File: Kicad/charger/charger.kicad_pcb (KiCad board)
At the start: 2 copper layers, 78 x 57 mm, 21 parts, among them K1 9V / 1A, K2 Battery, Q1 STN790A, U1 BQ2057W

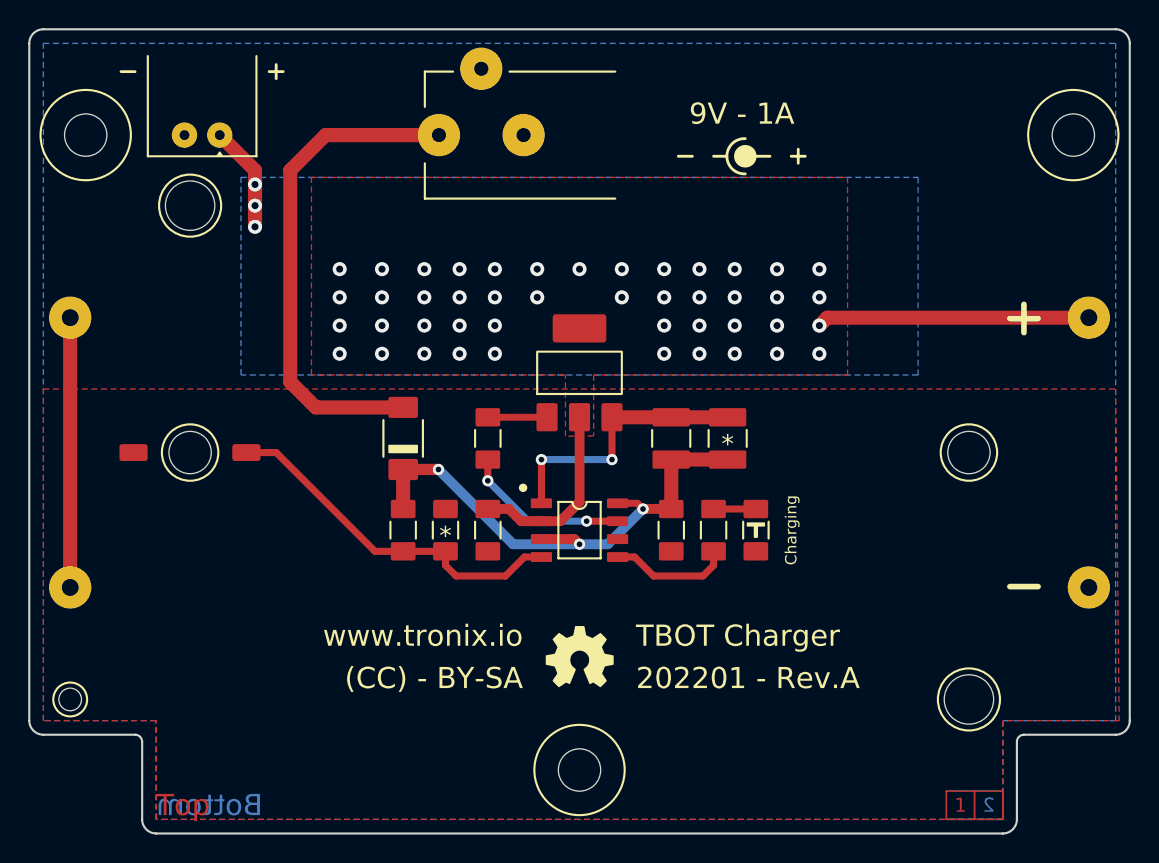
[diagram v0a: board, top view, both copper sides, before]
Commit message: Update
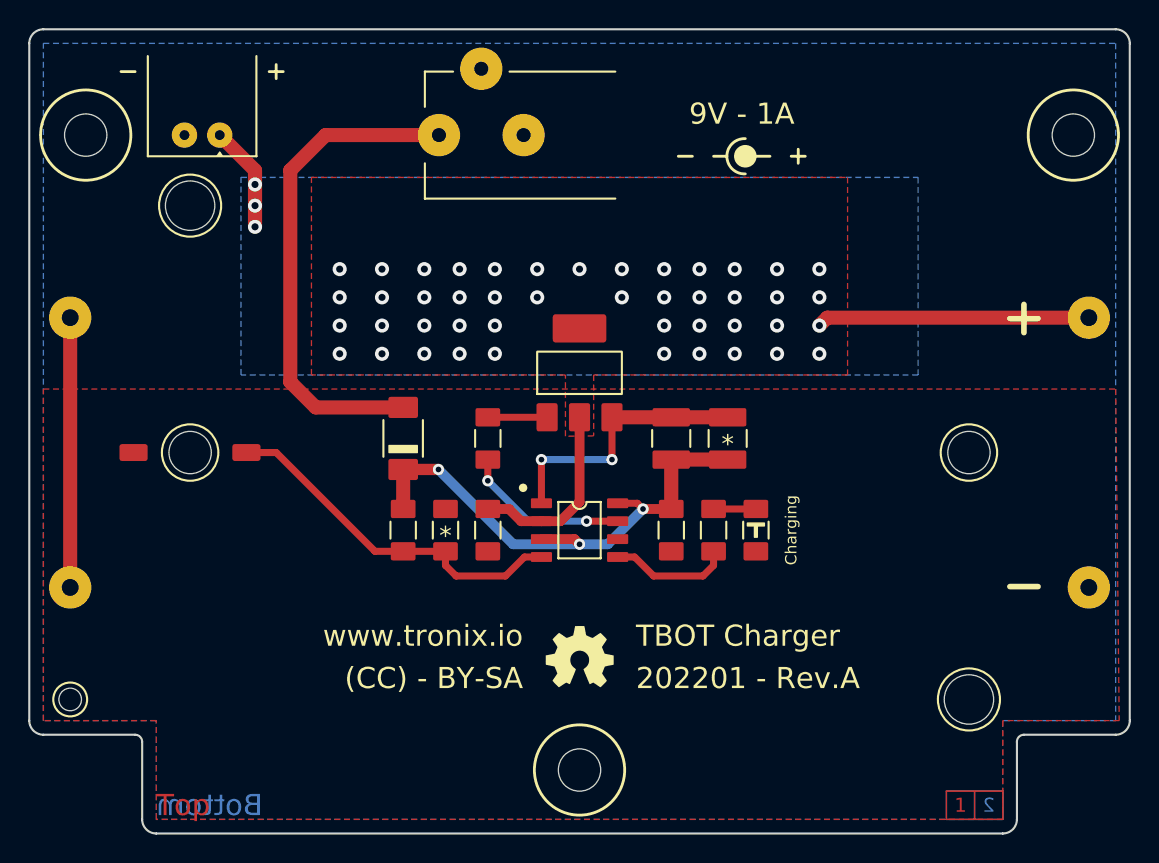
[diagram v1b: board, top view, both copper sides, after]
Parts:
- LED1: value PURPLE -> Charging
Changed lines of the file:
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@@
     (zone_connect 2)
     (attr smd)
-    (fp_text reference "D1" (at 4 0 90) (layer "F.Fab")
-        (effects (font (size 1 1) (thickness 0.15)))
-    )
-    (fp_text value "PMEG3030" (at 0 -2.5 90) (layer "F.Fab")
+    (fp_text reference "D1" (at 0 0 90) (layer "F.SilkS") hide
+        (effects (font (size 1 1) (thickness 0.15)))
+    )
+    (fp_text value "PMEG3030" (at 0 2.5 90) (layer "F.Fab")
         (effects (font (size 1 1) (thickness 0.15)))
     )
@@
     (zone_connect 2)
     (attr smd)
-    (fp_text reference "R6" (at 0 -2 -90) (layer "F.Fab")
+    (fp_text reference "R6" (at 0 -2 -90) (layer "F.SilkS") hide
         (effects (font (size 1 1) (thickness 0.15)))
     )
@@
     (zone_connect 2)
     (attr smd)
-    (fp_text reference "R5" (at 0 -2 90) (layer "F.Fab")
+    (fp_text reference "R5" (at 0 -2 90) (layer "F.SilkS") hide
         (effects (font (size 1 1) (thickness 0.15)))
     )
@@
     (property "ki_description" "Unpolarized Capacitor")
     (attr smd)
-    (fp_text reference "C1" (at 0 -2 -90) (layer "F.Fab")
+    (fp_text reference "C1" (at 0 -2 -90) (layer "F.SilkS") hide
         (effects (font (size 1 1) (thickness 0.15)))
     )
@@
     (zone_connect 2)
     (attr smd)
-    (fp_text reference "R1" (at 0 -2 -90) (layer "F.Fab")
+    (fp_text reference "R1" (at 0 -2 -90) (layer "F.SilkS") hide
         (effects (font (size 1 1) (thickness 0.15)))
     )
@@
     (property "ki_description" "DC Barrel Jack with an Internal Switch")
     (attr through_hole)
-    (fp_text reference "K1" (at 1 5.4625 180) (layer "F.Fab")
-        (effects (font (size 1 1) (thickness 0.15)))
-    )
-    (fp_text value "9V / 1A" (at -1 5.4625 180) (layer "F.Fab")
+    (fp_text reference "K1" (at 0 -2.5 90) (layer "F.SilkS") hide
+        (effects (font (size 1 1) (thickness 0.15)))
+    )
+    (fp_text value "9V / 1A" (at 0 15 90) (layer "F.Fab")
         (effects (font (size 1 1) (thickness 0.15)))
     )
@@
     (property "ki_description" "Unpolarized Capacitor")
     (attr smd)
-    (fp_text reference "C2" (at 0 -2 -90) (layer "F.Fab")
+    (fp_text reference "C2" (at 0 -2 -90) (layer "F.SilkS") hide
         (effects (font (size 1 1) (thickness 0.15)))
     )
@@
     (property "ki_description" "Medium current, high performance, low voltage PNP transistor")
     (attr smd)
-    (fp_text reference "Q1" (at 0 0 180) (layer "F.Fab")
-        (effects (font (size 1 1) (thickness 0.15)))
-    )
-    (fp_text value "STN790A" (at -4 0 180) (layer "F.Fab")
+    (fp_text reference "Q1" (at 0 -4.5 90) (layer "F.SilkS") hide
+        (effects (font (size 1 1) (thickness 0.15)))
+    )
+    (fp_text value "STN790A" (at 0 4.5 90) (layer "F.Fab")
         (effects (font (size 1 1) (thickness 0.15)))
     )
@@
     (property "ki_description" "Resistor")
     (attr smd)
-    (fp_text reference "R2" (at 0 -2.5 90) (layer "F.Fab")
+    (fp_text reference "R2" (at 0 -2.5 90) (layer "F.SilkS") hide
         (effects (font (size 1 1) (thickness 0.15)))
     )
@@
     (zone_connect 2)
     (attr smd)
-    (fp_text reference "TH1" (at 0 -3.81 180) (layer "F.Fab")
-        (effects (font (size 1 1) (thickness 0.15)))
-    )
-    (fp_text value "10k" (at 0 3.81 180) (layer "F.Fab")
+    (fp_text reference "TH1" (at 0 -3 180) (layer "F.SilkS") hide
+        (effects (font (size 1 1) (thickness 0.15)))
+    )
+    (fp_text value "10k" (at 0 3 180) (layer "F.Fab")
         (effects (font (size 1 1) (thickness 0.15)))
     )
@@
     (zone_connect 2)
     (attr smd)
-    (fp_text reference "LED1" (at 0 -2 90) (layer "F.Fab")
-        (effects (font (size 1 1) (thickness 0.15)))
-    )
-    (fp_text value "PURPLE" (at 0 2 90) (layer "F.Fab")
+    (fp_text reference "LED1" (at 0 -2 90) (layer "F.SilkS") hide
+        (effects (font (size 1 1) (thickness 0.15)))
+    )
+    (fp_text value "Charging" (at 0 2 90) (layer "F.Fab")
         (effects (font (size 1 1) (thickness 0.15)))
     )
@@
     (property "ki_keywords" "538-22-05-7025 / 538-50-37-5023 / 538-08-70-1039-CT")
     (attr through_hole)
-    (fp_text reference "K2" (at -0.5 -4.5) (layer "F.Fab")
-        (effects (font (size 1 1) (thickness 0.15)))
-    )
-    (fp_text value "Battery" (at -0.5 -3) (layer "F.Fab")
+    (fp_text reference "K2" (at -1.5 -8) (layer "F.SilkS") hide
+        (effects (font (size 1 1) (thickness 0.15)))
+    )
+    (fp_text value "Battery" (at -1.5 3) (layer "F.Fab")
+        (effects (font (size 1 1) (thickness 0.15)))
+    )
+    (fp_text user "1" (at 2 0.2) (layer "F.Fab")
         (effects (font (size 1 1) (thickness 0.15)))
     )
     (fp_text user "${REFERENCE}" (at -1.25 -8) (layer "F.Fab")
-        (effects (font (size 1 1) (thickness 0.15)))
-    )
-    (fp_text user "1" (at 1.9 0.1 unlocked) (layer "F.Fab")
         (effects (font (size 1 1) (thickness 0.15)))
     )
@@
     (property "ki_description" "Resistor")
     (attr smd)
-    (fp_text reference "R3" (at 0 -2.5 90) (layer "F.Fab")
+    (fp_text reference "R3" (at 0 -2.5 90) (layer "F.SilkS") hide
         (effects (font (size 1 1) (thickness 0.15)))
     )
@@
     (property "ki_description" "Low Dropout linear 2-cell Li-ion charge controller with AutoCompTM, 8.4V")
     (attr smd)
-    (fp_text reference "U1" (at 0 -3.4) (layer "F.Fab")
-        (effects (font (size 1 1) (thickness 0.15)))
-    )
-    (fp_text value "BQ2057W" (at 0 3.4) (layer "F.Fab")
+    (fp_text reference "U1" (at 0 -3.5) (layer "F.SilkS") hide
+        (effects (font (size 1 1) (thickness 0.15)))
+    )
+    (fp_text value "BQ2057W" (at 0 3.5) (layer "F.Fab")
         (effects (font (size 1 1) (thickness 0.15)))
     )
@@
     (zone_connect 2)
     (attr smd)
-    (fp_text reference "R4" (at 0 -2 90) (layer "F.Fab")
+    (fp_text reference "R4" (at 0 -2 90) (layer "F.SilkS") hide
         (effects (font (size 1 1) (thickness 0.15)))
     )
@@
     (property "Sheetfile" "charger.kicad_sch")
     (property "Sheetname" "")
-    (attr exclude_from_pos_files)
-    (fp_text reference "H3" (at 0 4.2) (layer "B.Fab") hide
+    (attr exclude_from_pos_files exclude_from_bom)
+    (fp_text reference "H3" (at 0 4.5) (layer "B.Fab") hide
         (effects (font (size 1 1) (thickness 0.15)) (justify mirror))
     )
-    (fp_text value "MOUNTING-HOLE-3MM-MASK" (at 0 -4.2) (layer "B.Fab") hide
+    (fp_text value "MOUNTING-HOLE-3MM-MASK" (at 0 -4.5) (layer "B.Fab") hide
         (effects (font (size 1 1) (thickness 0.15)) (justify mirror))
     )
     (fp_circle (center 0 0) (end 3.2 0)
-      (stroke (width 0.15) (type solid)) (fill none) (layer "B.SilkS"))
+      (stroke (width 0.2) (type solid)) (fill none) (layer "B.SilkS"))
     (fp_circle (center 0 0) (end 3.2 0)
-      (stroke (width 0.15) (type solid)) (fill none) (layer "F.SilkS"))
+      (stroke (width 0.2) (type solid)) (fill none) (layer "F.SilkS"))
     (fp_circle (center 0 0) (end 3.2 0)
       (stroke (width 0.05) (type solid)) (fill none) (layer "B.CrtYd"))
@@
     (property "Sheetfile" "charger.kicad_sch")
     (property "Sheetname" "")
-    (attr exclude_from_pos_files)
-    (fp_text reference "H1" (at 0 4.2 270) (layer "B.Fab") hide
+    (attr exclude_from_pos_files exclude_from_bom)
+    (fp_text reference "H1" (at 0 4.5 270) (layer "B.Fab") hide
         (effects (font (size 1 1) (thickness 0.15)) (justify mirror))
     )
-    (fp_text value "MOUNTING-HOLE-3MM-MASK" (at 0 -4.2 270) (layer "B.Fab") hide
+    (fp_text value "MOUNTING-HOLE-3MM-MASK" (at 0 -4.5 270) (layer "B.Fab") hide
         (effects (font (size 1 1) (thickness 0.15)) (justify mirror))
     )
     (fp_circle (center 0 0) (end 3.2 0)
-      (stroke (width 0.15) (type solid)) (fill none) (layer "B.SilkS"))
+      (stroke (width 0.2) (type solid)) (fill none) (layer "B.SilkS"))
     (fp_circle (center 0 0) (end 3.2 0)
-      (stroke (width 0.15) (type solid)) (fill none) (layer "F.SilkS"))
+      (stroke (width 0.2) (type solid)) (fill none) (layer "F.SilkS"))
     (fp_circle (center 0 0) (end 3.2 0)
       (stroke (width 0.05) (type solid)) (fill none) (layer "B.CrtYd"))
@@
     (property "Sheetfile" "charger.kicad_sch")
     (property "Sheetname" "")
-    (attr exclude_from_pos_files)
-    (fp_text reference "H2" (at 0 4.2 270) (layer "B.Fab") hide
+    (attr exclude_from_pos_files exclude_from_bom)
+    (fp_text reference "H2" (at 0 4.5 270) (layer "B.Fab") hide
         (effects (font (size 1 1) (thickness 0.15)) (justify mirror))
     )
-    (fp_text value "MOUNTING-HOLE-3MM-MASK" (at 0 -4.2 270) (layer "B.Fab") hide
+    (fp_text value "MOUNTING-HOLE-3MM-MASK" (at 0 -4.5 270) (layer "B.Fab") hide
         (effects (font (size 1 1) (thickness 0.15)) (justify mirror))
     )
     (fp_circle (center 0 0) (end 3.2 0)
-      (stroke (width 0.15) (type solid)) (fill none) (layer "B.SilkS"))
+      (stroke (width 0.2) (type solid)) (fill none) (layer "B.SilkS"))
     (fp_circle (center 0 0) (end 3.2 0)
-      (stroke (width 0.15) (type solid)) (fill none) (layer "F.SilkS"))
+      (stroke (width 0.2) (type solid)) (fill none) (layer "F.SilkS"))
     (fp_circle (center 0 0) (end 3.2 0)
       (stroke (width 0.05) (type solid)) (fill none) (layer "B.CrtYd"))
@@
     (property "ki_description" "THM Holder for Dual 18650 Batteries")
     (attr through_hole)
-    (fp_text reference "BT1" (at 1 0 180) (layer "B.Fab")
+    (fp_text reference "BT1" (at 0 2 270) (layer "B.SilkS") hide
         (effects (font (size 1 1) (thickness 0.15)) (justify mirror))
     )
-    (fp_text value "18650" (at -1 0 180) (layer "B.Fab")
+    (fp_text value "18650" (at 0 -2 270) (layer "B.Fab")
         (effects (font (size 1 1) (thickness 0.15)) (justify mirror))
     )
